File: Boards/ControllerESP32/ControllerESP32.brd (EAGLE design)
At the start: 74.9 x 79.7 mm, 12 parts, among them J1 POWER_JACKPTH_BREAD

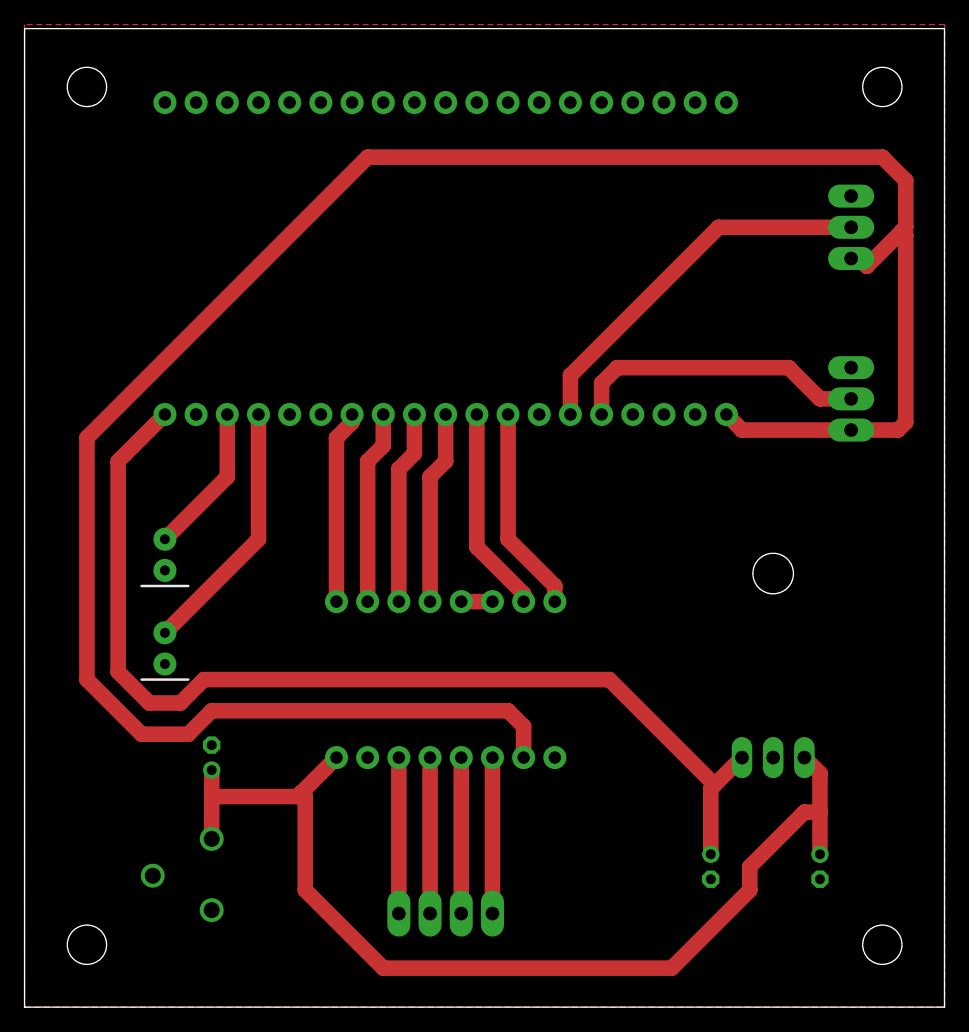
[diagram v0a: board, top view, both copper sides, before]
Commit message: finished esp32 board based board
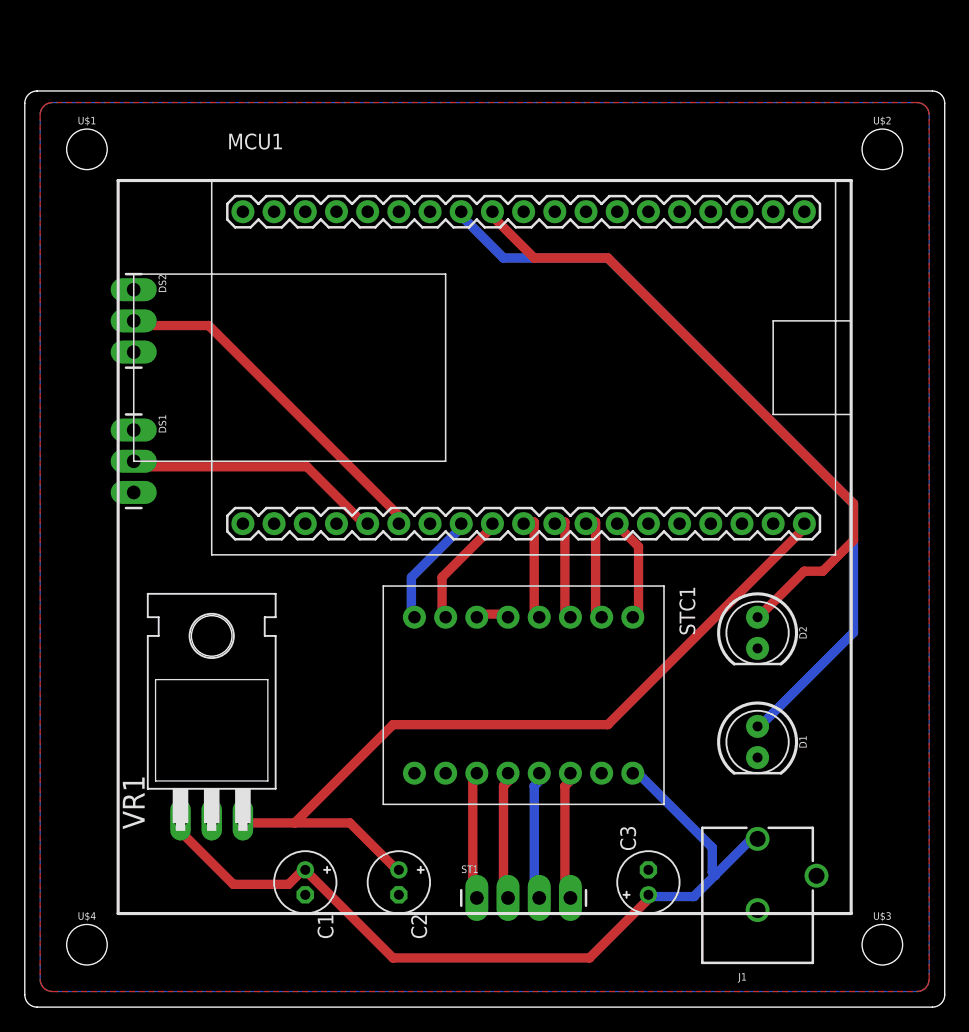
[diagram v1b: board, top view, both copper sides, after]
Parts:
- added U$1, U$2, U$3, U$4: (no value), SparkFun-Hardware:STAND-OFF
- moved DS2 58.9 mm to (8.89, 58.4), flipped to the top
- moved DS1 58.6 mm to (8.89, 47.0), flipped to the top
- moved D1 48.9 mm to (59.7, 21.6), flipped to the top
- moved D2 48.7 mm to (59.7, 30.5), flipped to the top
- moved VR1 46.0 mm to (15.2, 25.4), flipped to the top
- moved J1 44.4 mm to (59.7, 0.00), flipped to the top
- moved C1 41.9 mm to (22.9, 10.2), flipped to the top
- moved C3 37.0 mm to (50.8, 10.2), flipped to the top
- moved C2 25.4 mm to (30.5, 10.2), flipped to the top
- moved MCU1 10.9 mm to (40.6, 52.1), flipped to the top
- moved STC1 6.48 mm to (40.6, 25.4), flipped to the top
- moved ST1 1.80 mm to (36.8, 8.89), flipped to the top
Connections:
- net LED1: now also MCU1.31; no longer MCU1.16
- net LED2: now also MCU1.30; no longer MCU1.17
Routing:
- net 3V: track 178.8 -> 0.00 mm
- net LED1: track 20.9 -> 63.5 mm
- net LED2: track 12.3 -> 52.9 mm
- net 5V: track 85.4 -> 66.2 mm
- net 12V: track 84.5 -> 69.3 mm
- net STC_DIR: track 16.8 -> 9.39 mm
- net STC_STEP: track 16.8 -> 9.42 mm
- net STC_EN: track 15.8 -> 8.59 mm
- net STC_MS1: track 15.8 -> 8.86 mm
- net STC_MS2: track 15.8 -> 8.86 mm
- net STC_MS3: track 15.8 -> 8.86 mm
- net DS1_SIG: track 24.4 -> 21.3 mm
- net ST_BLUE: track 12.7 -> 10.7 mm
- net ST_YELLOW: track 12.7 -> 10.7 mm
- net ST_RED: track 12.7 -> 10.7 mm
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- added copper zone on layer 1, net 3V
- added copper zone on layer 16, net GND
- removed copper zone on layer 1, net GND
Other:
- board size 74.9 x 79.7 mm -> 74.9 x 74.6 mm
